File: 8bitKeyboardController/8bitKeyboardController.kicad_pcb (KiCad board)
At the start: 2 copper layers, 43.5 x 70 mm, 10 parts

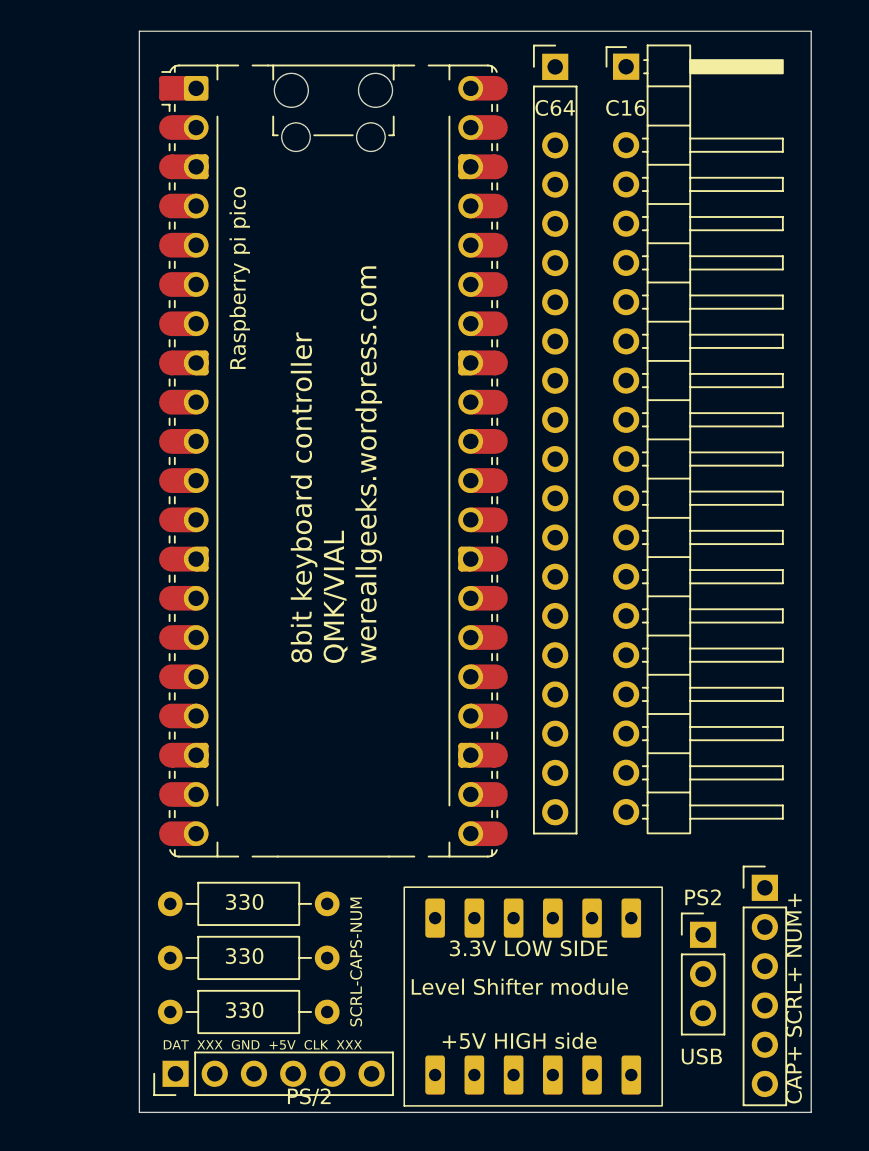
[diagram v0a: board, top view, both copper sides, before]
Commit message: PCB 1st routing
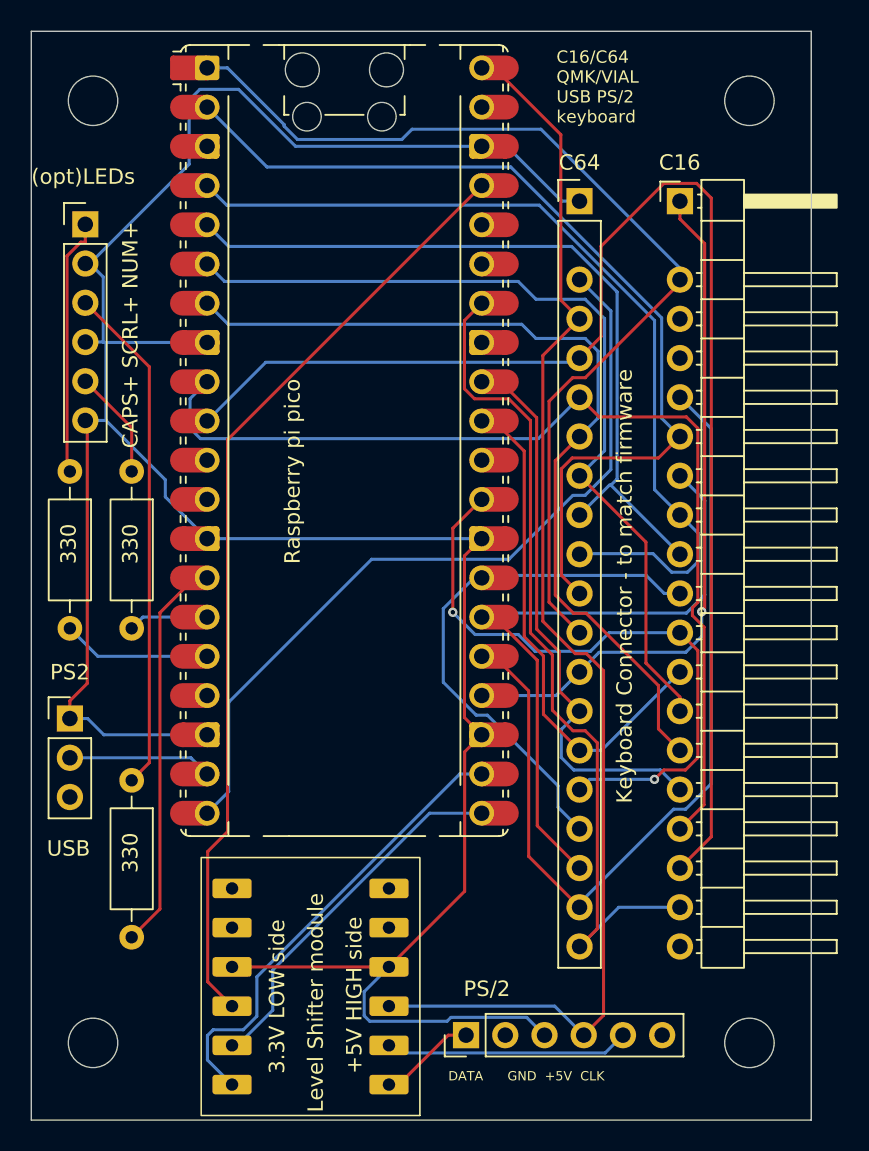
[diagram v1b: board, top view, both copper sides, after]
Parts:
- added G***: LOGO, LOGO, B.Cu at (152.5, 83.5)
- added HOLE-BOTTOMLEFT: MountingHole_3.2mm_M3, MountingHole:MountingHole_3.2mm_M3, F.Cu at (122.5, 116.0)
- added HOLE-BOTTOMRIGHT: MountingHole_3.2mm_M3, MountingHole:MountingHole_3.2mm_M3, F.Cu at (165.0, 116.0)
- added HOLE-TOPLEFT: MountingHole_3.2mm_M3, MountingHole:MountingHole_3.2mm_M3, F.Cu at (122.5, 55.0)
- added HOLE-TOPRIGHT: MountingHole_3.2mm_M3, MountingHole:MountingHole_3.2mm_M3, F.Cu at (165.0, 55.0)
- moved LEDS(opt)1 61.5 mm to (122.0, 63.0)
- moved PS2 43.3 mm to (121.0, 95.0)
- moved RCAPS1 31.6 mm to (125.0, 79.0), turned to -90 degrees
- moved RNUM1 28.7 mm to (121.0, 79.0), turned to -90 degrees
- moved PS/2 19.0 mm to (146.7, 115.5)
- moved RSCROLL1 15.2 mm to (125.0, 99.0), turned to -90 degrees
- moved C16 9.38 mm to (160.5, 61.5)
- moved C64 8.84 mm to (154.0, 61.5)
- moved LVL1 3.05 mm to (141.7, 118.7), turned to 180 degrees
- moved Raspberry_Pi_Pico1 1.50 mm to (138.8, 77.0)
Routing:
- net Net-(C64-Pin_1): track 0.00 -> 183.4 mm
- net Net-(C16-Pin_18): track 0.00 -> 87.9 mm
- net Net-(C64-Pin_4): track 0.00 -> 82.7 mm
- net Net-(C16-Pin_17): track 0.00 -> 66.4 mm
- net Net-(C16-Pin_3): track 0.00 -> 65.8 mm
- net Net-(LVL1-LV): track 0.00 -> 61.9 mm
- net Net-(C16-Pin_7): track 0.00 -> 61.2 mm
- net Net-(C16-Pin_9): track 0.00 -> 58.7 mm
- net Net-(C16-Pin_15): track 0.00 -> 58.2 mm
- net Net-(C16-Pin_6): track 0.00 -> 57.2 mm
- net Net-(C16-Pin_14): track 0.00 -> 56.8 mm
- net Net-(C16-Pin_19): track 0.00 -> 56.3 mm
- net Net-(C64-Pin_3): track 0.00 -> 52.7 mm
- net Net-(C16-Pin_10): track 0.00 -> 51.0 mm
- net Net-(C16-Pin_1): track 0.00 -> 45.5 mm, vias 0 -> 1
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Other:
- board size 43.5 x 70 mm -> 50.5 x 70.5 mm
- board text added: "(opt)LEDs"
- board text added: "2026/09/24"
- board text added: "3.3V LOW side"
- board text added: "C16/C64 Keyboard QMK/VIAL USB PS/2"
- board text added: "C16/C64 QMK/VIAL Keyboard Controller PCB"
- board text added: "C16/C64 QMK/VIAL USB PS/2 keyboard"
- board text added: "CAPS+ SCRL+ NUM+"
- board text added: "DATA GND +5V CLK"
- board text added: "Geeky keyboard controller board"
- board text added: "Keyboard Connector - to match firmware"
- board text added: "wereallgeeks.wordpress.com"
- board text removed: "3.3V LOW SIDE"
- board text removed: "8bit keyboard controller QMK/VIAL wereallgeeks.wordpress.com"
- board text removed: "CAP+ SCRL+ NUM+"
- board text removed: "DAT XXX GND +5V CLK XXX"
- board text removed: "SCRL-CAPS-NUM"
